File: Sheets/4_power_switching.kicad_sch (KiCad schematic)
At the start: 34 parts, among them Q2 SSM3J332R, Q3 SSM3J332R, U4 TP6841S6, U5 MIC5205-3.3YM5

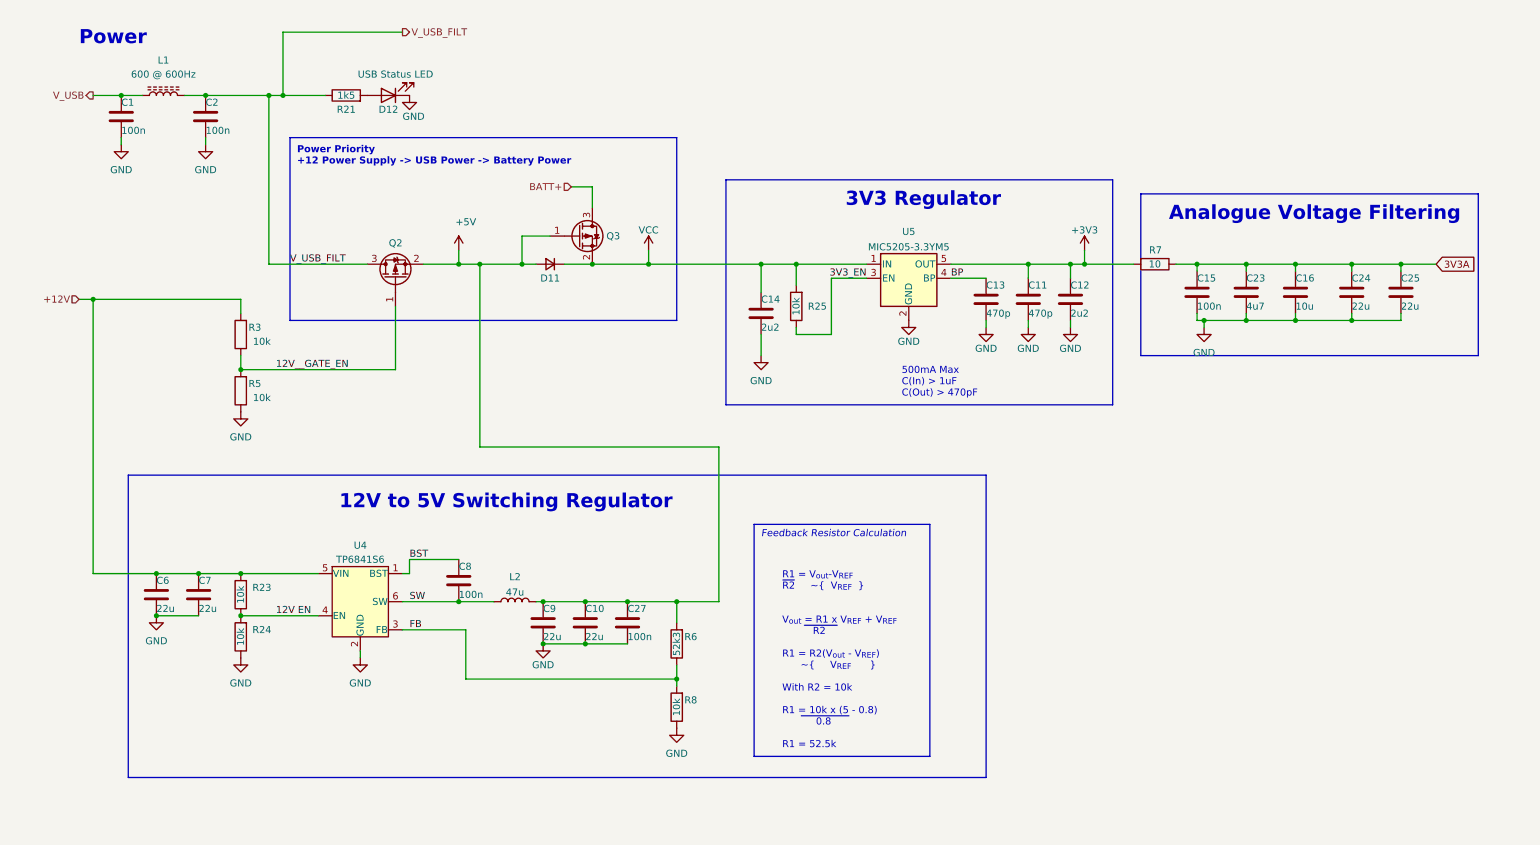
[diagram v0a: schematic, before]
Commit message: Updates for revision 2
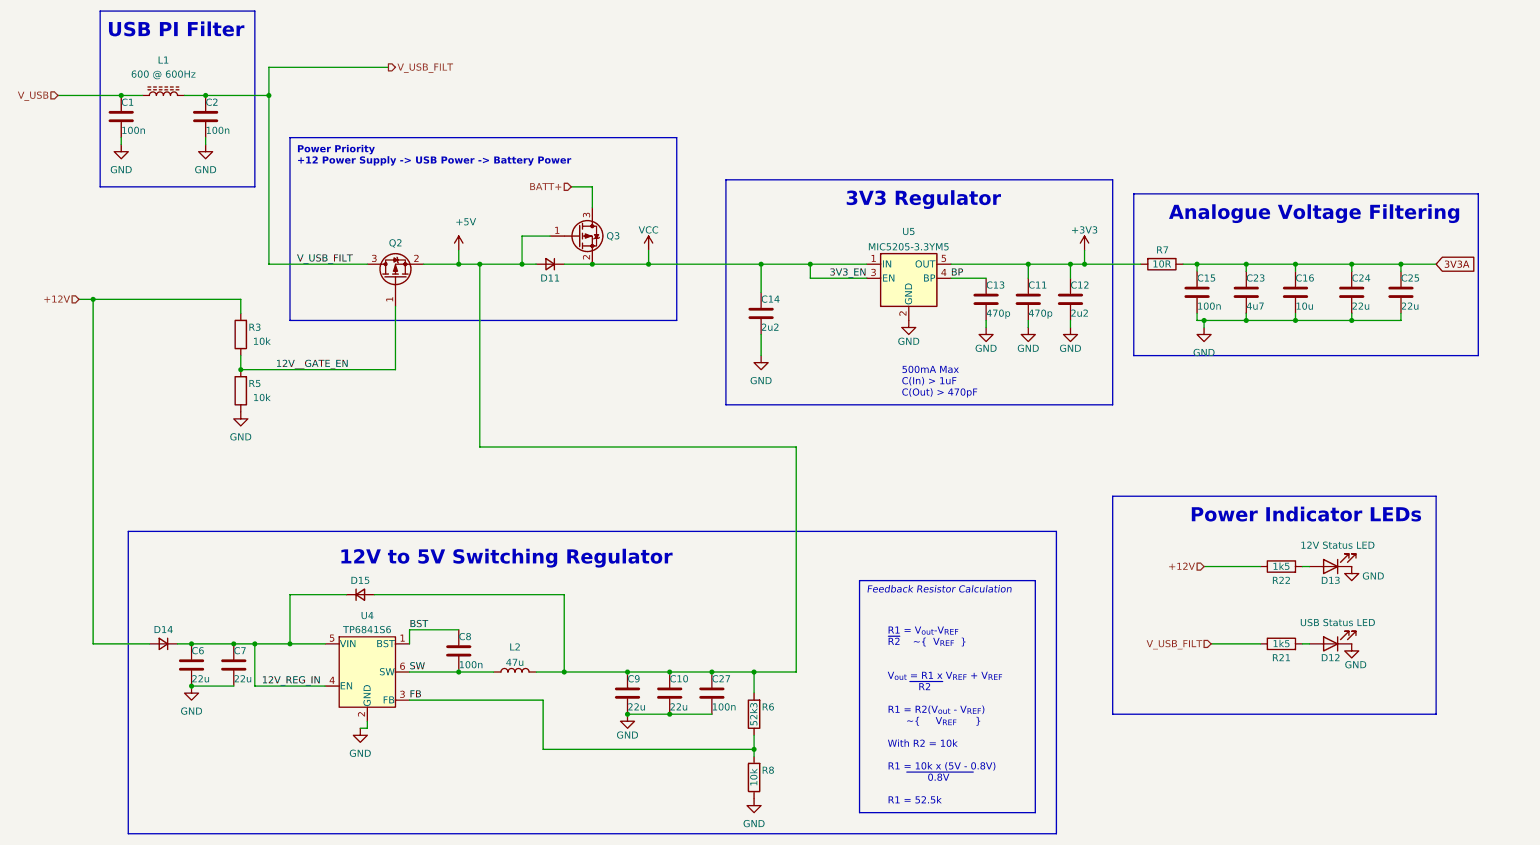
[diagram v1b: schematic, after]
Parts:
- removed R23, R24, R25: 10k, Resistor_SMD:R_0402_1005Metric, symbol Device:R
- added D13: 12V Status LED, LED_SMD:LED_0805_2012Metric, symbol Device:LED
- added D14, D15: D_Small, Diode_SMD:D_SOD-123F, symbol Device:D_Small
- added R22: 1k5, Resistor_SMD:R_0402_1005Metric, symbol Device:R
- C10, C24, C25, C6, C7, C9: MANUFACTURER (none) -> Murata Electronics; MAXIMUM_PACKAGE_HEIGHT Murata Electronics -> (none)
- D11: MANUFACTURER (none) -> LRC; MAXIMUM_PACKAGE_HEIGHT LRC -> (none)
- R7: value 10 -> 10R
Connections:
- net 3V3_EN is gone; now on net VCC: U5.3 (EN)
- net +12V: now also D14.2 (A), R22.1; no longer C6.1, C7.1, U4.5 (VIN)
- net +5V: now also D15.2 (A)
- net GND: now also D13.1 (K)
- net 12V EN renamed 12V_REG_IN
- net 12V_REG_IN: now also C6.1, C7.1, U4.5 (VIN), D14.1 (K), D15.1 (K)
- new net: D13.2 (A), R22.2
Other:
- note added: "Power Indicator LEDs"
- note added: "R1 = V_{out}-V_{REF} ~{R2} ~{ V_{REF} } V_{out} = R1 x V_{REF} + V_{REF} ~{ R2 } R1 = R2(V_{out} - V_{REF}) ~{ V_{REF} } With R2 = 10k R1 = 10k x (5V - 0.8V) ~{ 0.8V } R1 = 52.5k"
- note added: "USB PI Filter"
- note removed: "Power"
- note removed: "R1 = V_{out}-V_{REF} ~{R2} ~{ V_{REF} } V_{out} = R1 x V_{REF} + V_{REF} ~{ R2 } R1 = R2(V_{out} - V_{REF}) ~{ V_{REF} } With R2 = 10k R1 = 10k x (5 - 0.8) ~{ 0.8 } R1 = 52.5k"
- moved on the sheet: C10, C27, C6, C7, C8, C9, L2, R6, R7, R8, U4

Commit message: Updating bom with datasheets, manufactures, and part numbers
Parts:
- C1, C12, C14, C15, C16, C2, C23, C27, C8: MANUFACTURER (none) -> Samsung Electro-Mechanics
- C11, C13: MANUFACTURER (none) -> FH (Guangdong Fenghua Advanced Tech)
- D12, D13: MANUFACTURER (none) -> Orient
- L1, L2: MANUFACTURER (none) -> Sunlord
- Q2, Q3: Manufacturer Part Number SSM3J332R -> SSM3J332R,LF
- U4: MANUFACTURER (none) -> TECH PUBLIC
- U5: MANUFACTURER (none) -> Microchip Tech
